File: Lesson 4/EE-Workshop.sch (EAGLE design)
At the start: 1 part

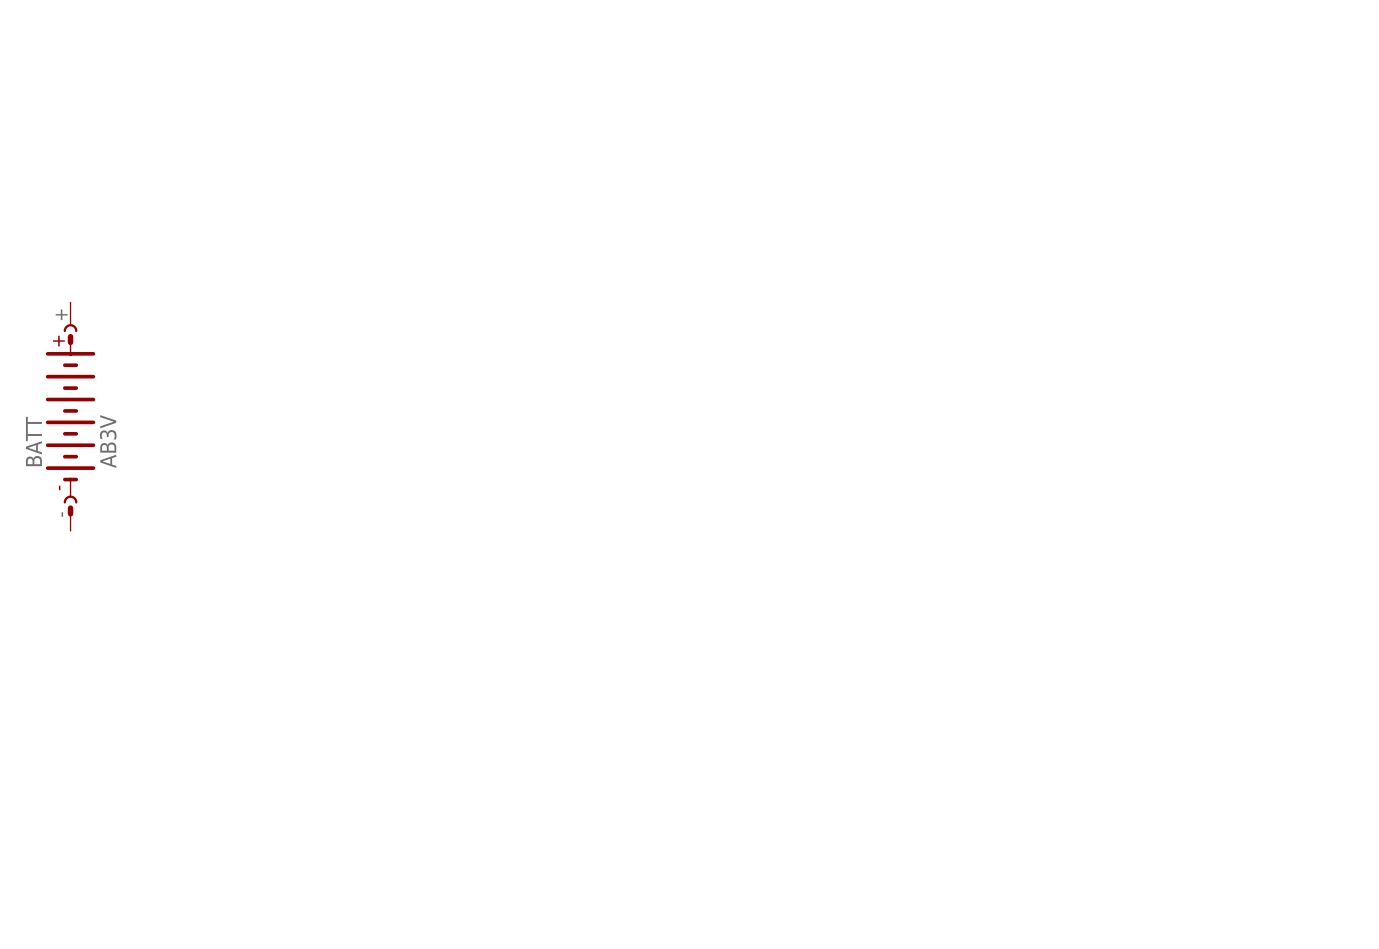
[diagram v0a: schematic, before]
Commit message: piano
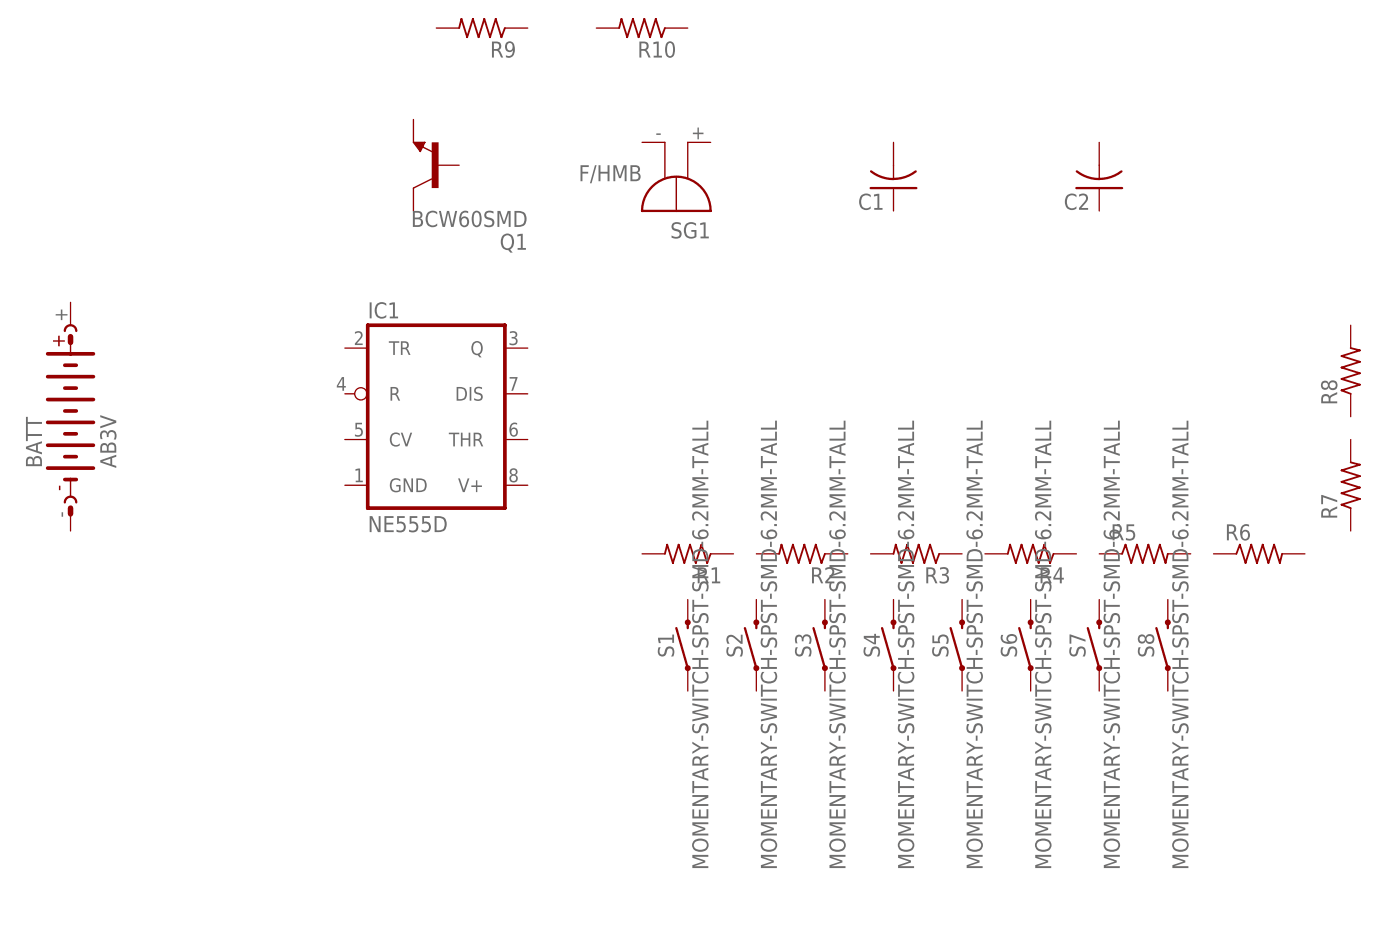
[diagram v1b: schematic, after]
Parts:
- added C1, C2: (no value), rcl:C-USC0805
- added IC1: NE555D, linear:NE555D
- added Q1: BCW60SMD, transistor-npn:BCW60SMD
- added R1, R10, R2, R3, R4, R5, R6, R7, R8, R9: (no value), rcl:R-US_R0805
- added S1, S2, S3, S4, S5, S6, S7, S8: MOMENTARY-SWITCH-SPST-SMD-6.2MM-TALL, SparkFun-Switches:MOMENTARY-SWITCH-SPST-SMD-6.2MM-TALL
- added SG1: F/HMB, buzzer:F/HMB
